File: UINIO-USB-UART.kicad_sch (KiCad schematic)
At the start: 36 parts, among them J1 Conn_01x08_Male, J2 Conn_01x04_Male, J3 Conn_01x07_Male, J4 Conn_01x06_Male, J5 Conn_01x04_Male, J6 Conn_01x07_Male, J7 Conn_01x03_Male, U1 CP2102, U2 CH343P

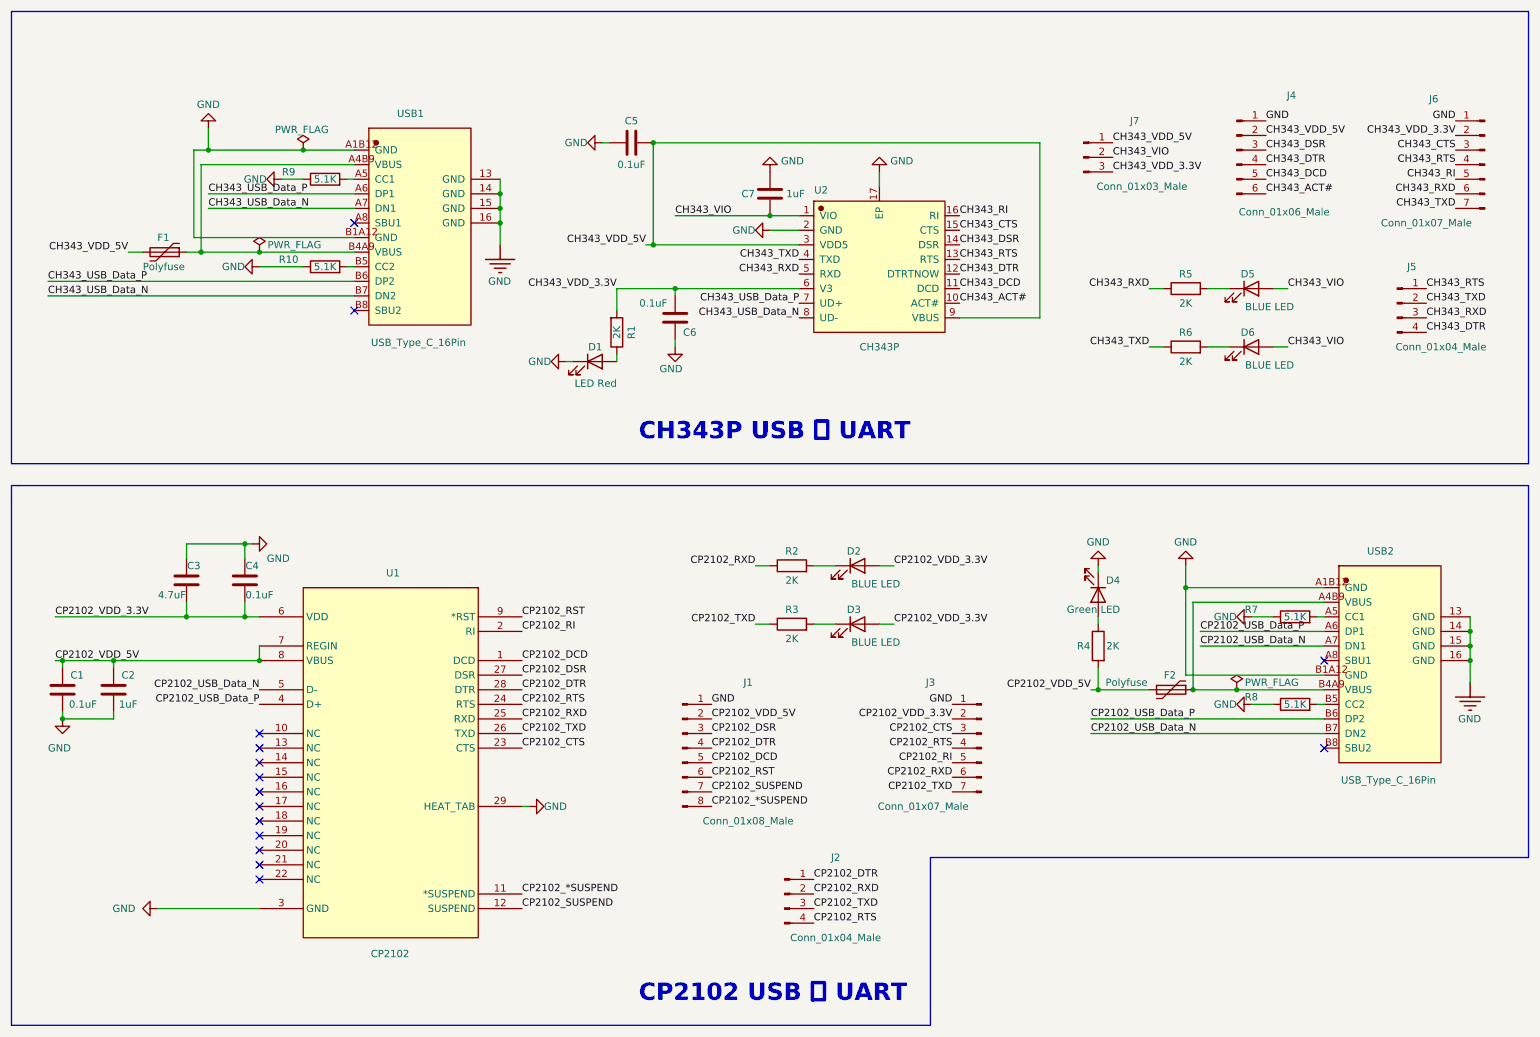
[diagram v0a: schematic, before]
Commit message: PCB Update.
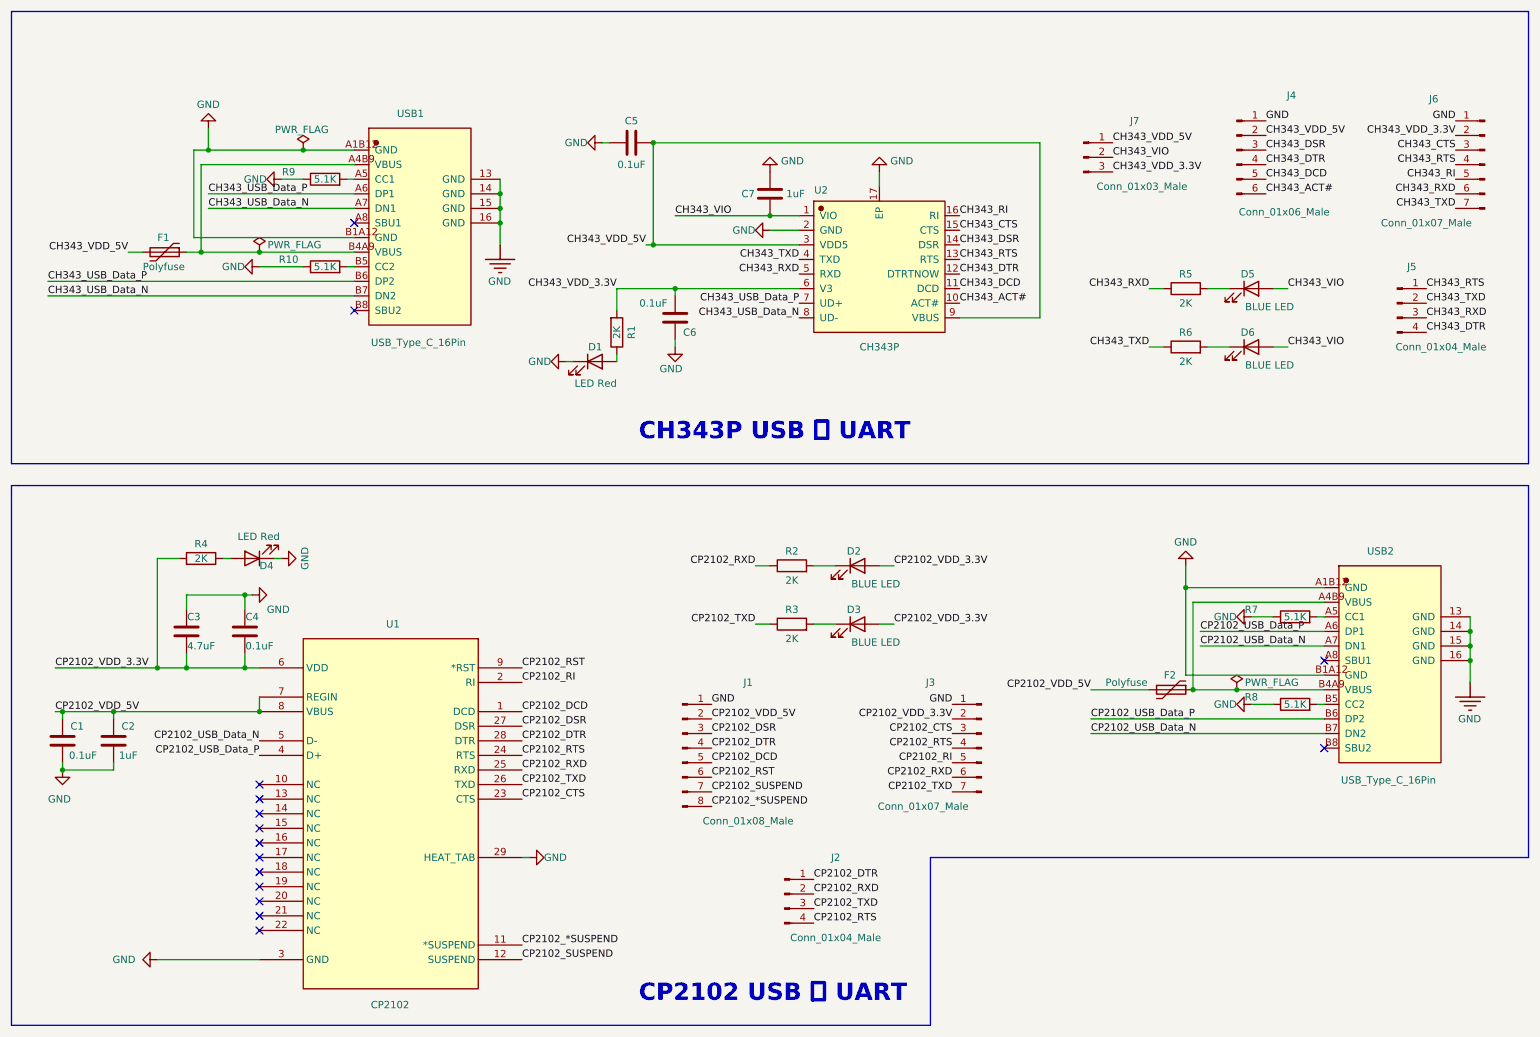
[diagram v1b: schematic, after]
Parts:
- D4: value Green LED -> LED Red
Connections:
- net CP2102_VDD_3.3V: now also R4.2
- net CP2102_VDD_5V: no longer R4.2
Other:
- moved on the sheet: C1, C2, C3, C4, D4, R4, U1
